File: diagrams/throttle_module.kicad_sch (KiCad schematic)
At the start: 5 parts, among them U1 MCU, U2 ADS1115, U3 Throttle, U4 Controller

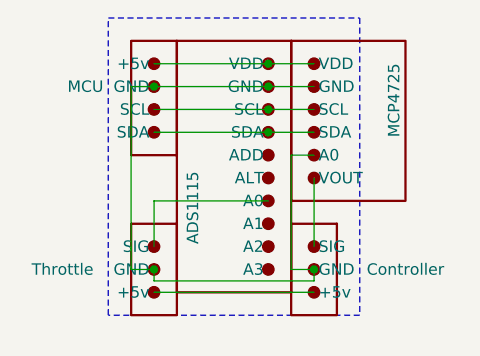
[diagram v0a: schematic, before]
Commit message: docs & diagrams
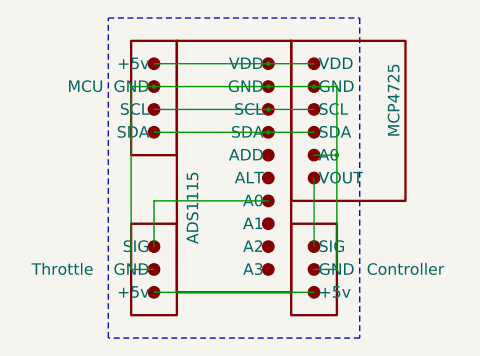
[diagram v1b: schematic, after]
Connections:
- net at U3. (SIG): now also U4. (SIG); no longer U2. (VDD)
- net at U4. (SIG): now also U?. (VOUT); no longer U3. (SIG)
- new net: U1. (SDA), U2. (VDD), U3. (SIG), U4. (SIG), U?. (VOUT)
- new net: U1. (SDA), U2. (VDD), U?. (VOUT) (x3)
- new net: U2. (VDD), U3. (SIG)
- now unconnected: U2. (VDD), U2. (VDD), U2. (VDD), U2. (VDD)
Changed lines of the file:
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@@
+	)
+	(junction
+		(at 93.98 48.26)
+		(diameter 0.5)
+		(color 0 0 0 1)
 	)
 	(junction
 		(at 86.36 45.72)
-		(diameter 0)
+		(diameter 0.5)
 		(color 194 194 0 1)
 	)
 	(junction
-		(at 91.44 60.96)
-		(diameter 0)
+		(at 86.36 40.64)
+		(diameter 0.5)
 		(color 0 0 0 1)
 	)
 	(junction
 		(at 86.36 38.1)
-		(diameter 0)
+		(diameter 0.5)
 		(color 194 0 0 1)
 	)
 	(junction
-		(at 86.36 40.64)
-		(diameter 0)
-		(color 0 0 0 1)
-	)
-	(junction
 		(at 86.36 43.18)
-		(diameter 0)
+		(diameter 0.5)
 		(color 255 153 0 1)
 	)
 	(junction
 		(at 73.66 40.64)
-		(diameter 0)
-		(color 0 0 0 1)
-	)
-	(junction
-		(at 73.66 60.96)
-		(diameter 0)
-		(color 0 0 0 1)
+		(diameter 0.5)
+		(color 0 0 0 1)
+	)
+	(junction
+		(at 91.44 40.64)
+		(diameter 0.5)
+		(color 0 0 0 1)
+	)
+	(wire
+		(pts
+			(xy 93.98 40.64) (xy 93.98 48.26)
+		)
+		(stroke
+			(width 0.2)
+			(type default)
+			(color 0 0 0 1)
+		)
 	)
 	(wire
@@
 		)
 		(stroke
-			(width 0)
+			(width 0.2)
 			(type default)
 		)
@@
 		)
 		(stroke
-			(width 0)
+			(width 0.2)
 			(type default)
 			(color 194 0 0 1)
@@
 		)
 		(stroke
-			(width 0)
+			(width 0.2)
 			(type default)
 			(color 194 194 0 1)
@@
 		)
 		(stroke
-			(width 0)
+			(width 0.2)
 			(type default)
 			(color 194 194 0 1)
@@
 	(wire
 		(pts
-			(xy 73.66 62.23) (xy 91.44 62.23)
-		)
-		(stroke
-			(width 0)
-			(type default)
-			(color 0 0 0 1)
-		)
-	)
-	(wire
-		(pts
-			(xy 91.44 62.23) (xy 91.44 60.96)
-		)
-		(stroke
-			(width 0)
+			(xy 86.36 40.64) (xy 91.44 40.64)
+		)
+		(stroke
+			(width 0.2)
+			(type default)
+			(color 0 0 0 1)
+		)
+	)
+	(wire
+		(pts
+			(xy 73.66 38.1) (xy 86.36 38.1)
+		)
+		(stroke
+			(width 0.2)
+			(type default)
+			(color 194 0 0 1)
+		)
+	)
+	(wire
+		(pts
+			(xy 93.98 60.96) (xy 93.98 48.26)
+		)
+		(stroke
+			(width 0.2)
 			(type default)
 			(color 0 0 0 1)
@@
 		)
 		(stroke
-			(width 0)
+			(width 0.2)
 			(type default)
 			(color 194 0 0 1)
@@
 	(wire
 		(pts
-			(xy 73.66 60.96) (xy 73.66 62.23)
-		)
-		(stroke
-			(width 0)
-			(type default)
-			(color 0 0 0 1)
-		)
-	)
-	(wire
-		(pts
-			(xy 73.66 38.1) (xy 86.36 38.1)
-		)
-		(stroke
-			(width 0)
-			(type default)
-			(color 194 0 0 1)
-		)
-	)
-	(wire
-		(pts
-			(xy 88.9 60.96) (xy 88.9 48.26)
-		)
-		(stroke
-			(width 0)
-			(type default)
-			(color 0 0 0 1)
-		)
-	)
-	(wire
-		(pts
 			(xy 91.44 50.8) (xy 91.44 58.42)
 		)
 		(stroke
-			(width 0)
-			(type default)
-		)
-	)
-	(wire
-		(pts
-			(xy 88.9 48.26) (xy 91.44 48.26)
-		)
-		(stroke
-			(width 0)
+			(width 0.2)
+			(type default)
+		)
+	)
+	(wire
+		(pts
+			(xy 93.98 48.26) (xy 91.44 48.26)
+		)
+		(stroke
+			(width 0.2)
 			(type default)
 			(color 0 0 0 1)
@@
 		)
 		(stroke
-			(width 0)
-			(type default)
-			(color 0 0 0 1)
-		)
-	)
-	(wire
-		(pts
-			(xy 71.12 60.96) (xy 71.12 40.64)
-		)
-		(stroke
-			(width 0)
+			(width 0.2)
 			(type default)
 			(color 0 0 0 1)
@@
 		)
 		(stroke
-			(width 0)
+			(width 0.2)
 			(type default)
 			(color 255 153 0 1)
@@
 	(wire
 		(pts
-			(xy 86.36 40.64) (xy 91.44 40.64)
-		)
-		(stroke
-			(width 0)
+			(xy 91.44 40.64) (xy 93.98 40.64)
+		)
+		(stroke
+			(width 0.2)
+			(type default)
+			(color 0 0 0 1)
+		)
+	)
+	(wire
+		(pts
+			(xy 71.12 60.96) (xy 73.66 60.96)
+		)
+		(stroke
+			(width 0.2)
 			(type default)
 			(color 0 0 0 1)
@@
 		)
 		(stroke
-			(width 0)
+			(width 0.2)
 			(type default)
 			(color 255 153 0 1)
@@
 		)
 		(stroke
-			(width 0)
-			(type default)
-			(color 0 0 0 1)
-		)
-	)
-	(wire
-		(pts
-			(xy 73.66 60.96) (xy 71.12 60.96)
-		)
-		(stroke
-			(width 0)
+			(width 0.2)
+			(type default)
+			(color 0 0 0 1)
+		)
+	)
+	(wire
+		(pts
+			(xy 71.12 40.64) (xy 71.12 60.96)
+		)
+		(stroke
+			(width 0.2)
 			(type default)
 			(color 0 0 0 1)
@@
 		)
 		(stroke
-			(width 0)
-			(type default)
-		)
-	)
-	(wire
-		(pts
-			(xy 91.44 60.96) (xy 88.9 60.96)
-		)
-		(stroke
-			(width 0)
+			(width 0.2)
+			(type default)
+		)
+	)
+	(wire
+		(pts
+			(xy 93.98 60.96) (xy 91.44 60.96)
+		)
+		(stroke
+			(width 0.2)
 			(type default)
 			(color 0 0 0 1)
@@
 	(rectangle
 		(start 68.58 33.02)
-		(end 96.52 66.04)
+		(end 96.52 68.58)
 		(stroke
 			(width 0)
